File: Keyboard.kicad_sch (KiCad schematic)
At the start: 166 parts, among them SW1 RotaryEncoder, U1 nice_nano

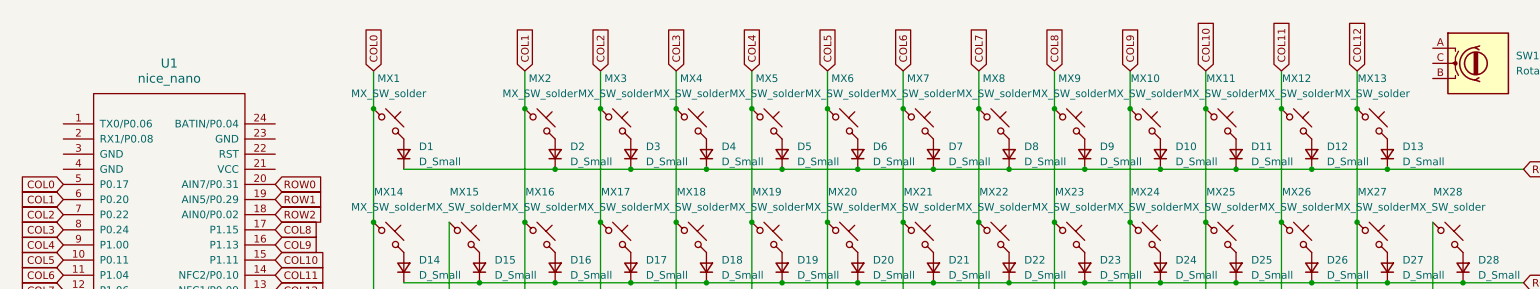
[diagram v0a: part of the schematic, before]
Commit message: project files
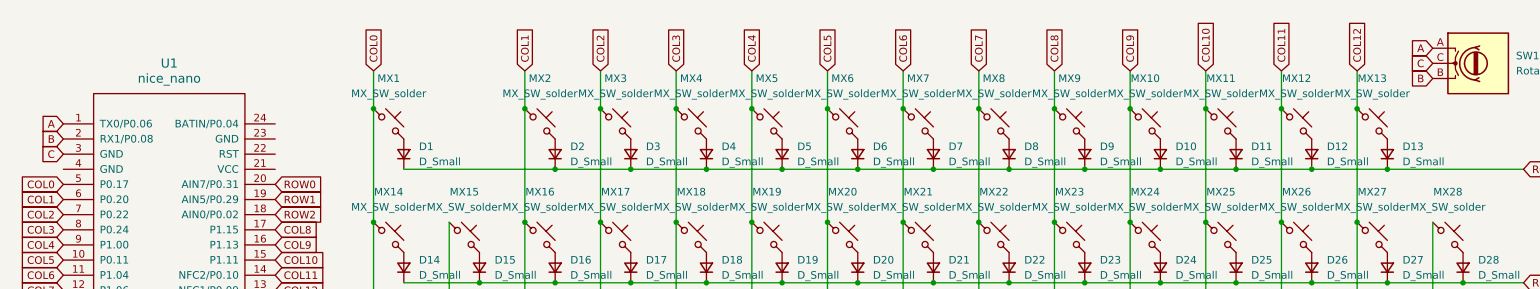
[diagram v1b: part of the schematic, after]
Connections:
- net A: now reaches U1.1 (TX0/P0.06)
- net A: now also SW1.A
- net B: now reaches U1.2 (RX1/P0.08)
- net B: now also SW1.B
- net C: now reaches U1.3 (GND)
- net C: now also SW1.C
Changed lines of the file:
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@@
+		)
+	)
+	(global_label "A"
+		(shape input)
+		(at 22.86 44.45 180)
+		(fields_autoplaced yes)
+		(effects
+			(font
+				(size 1.27 1.27)
+			)
+			(justify right)
+		)
+		(property "Intersheetrefs" "${INTERSHEET_REFS}"
+			(at 18.7862 44.45 0)
+			(effects
+				(font
+					(size 1.27 1.27)
+				)
+				(justify right)
+				(hide yes)
+			)
+		)
+	)
+	(global_label "B"
+		(shape input)
+		(at 252.73 36.83 180)
+		(fields_autoplaced yes)
+		(effects
+			(font
+				(size 1.27 1.27)
+			)
+			(justify right)
+		)
+		(property "Intersheetrefs" "${INTERSHEET_REFS}"
+			(at 248.4748 36.83 0)
+			(effects
+				(font
+					(size 1.27 1.27)
+				)
+				(justify right)
+				(hide yes)
+			)
 		)
 	)
@@
 		)
 	)
+	(global_label "C"
+		(shape input)
+		(at 22.86 49.53 180)
+		(fields_autoplaced yes)
+		(effects
+			(font
+				(size 1.27 1.27)
+			)
+			(justify right)
+		)
+		(property "Intersheetrefs" "${INTERSHEET_REFS}"
+			(at 18.6048 49.53 0)
+			(effects
+				(font
+					(size 1.27 1.27)
+				)
+				(justify right)
+				(hide yes)
+			)
+		)
+	)
 	(global_label "COL12"
 		(shape input)
@@
 		)
 	)
+	(global_label "B"
+		(shape input)
+		(at 22.86 46.99 180)
+		(fields_autoplaced yes)
+		(effects
+			(font
+				(size 1.27 1.27)
+			)
+			(justify right)
+		)
+		(property "Intersheetrefs" "${INTERSHEET_REFS}"
+			(at 18.6048 46.99 0)
+			(effects
+				(font
+					(size 1.27 1.27)
+				)
+				(justify right)
+				(hide yes)
+			)
+		)
+	)
 	(global_label "ROW4"
 		(shape input)
@@
 		)
 	)
+	(global_label "C"
+		(shape input)
+		(at 252.73 34.29 180)
+		(fields_autoplaced yes)
+		(effects
+			(font
+				(size 1.27 1.27)
+			)
+			(justify right)
+		)
+		(property "Intersheetrefs" "${INTERSHEET_REFS}"
+			(at 248.4748 34.29 0)
+			(effects
+				(font
+					(size 1.27 1.27)
+				)
+				(justify right)
+				(hide yes)
+			)
+		)
+	)
 	(global_label "COL2"
 		(shape input)
@@
 				(hide yes)
 			)
+		)
+	)
+	(global_label "A"
+		(shape input)
+		(at 252.73 31.75 180)
+		(fields_autoplaced yes)
+		(effects
+			(font
+				(size 1.27 1.27)
+			)
+			(justify right)
+		)
+		(property "Intersheetrefs" "${INTERSHEET_REFS}"
+			(at 248.6562 31.75 0)
+			(effects
+				(font
+					(size 1.27 1.27)
+				)
+				(justify right)
+				(hide yes)
+			)
